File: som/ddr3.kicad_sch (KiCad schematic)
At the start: 10 parts, among them U2 AS4C256M16D3, U3 AS4C256M16D3

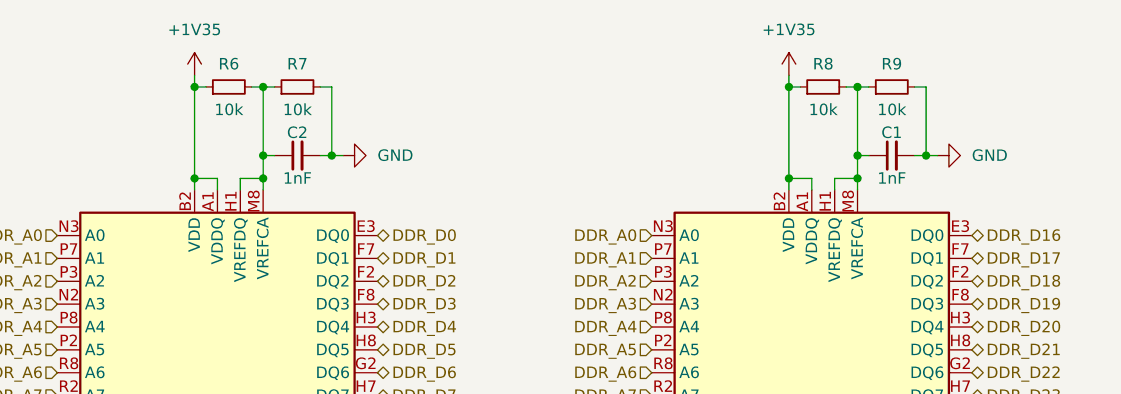
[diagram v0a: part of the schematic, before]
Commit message: DDR3 (again)
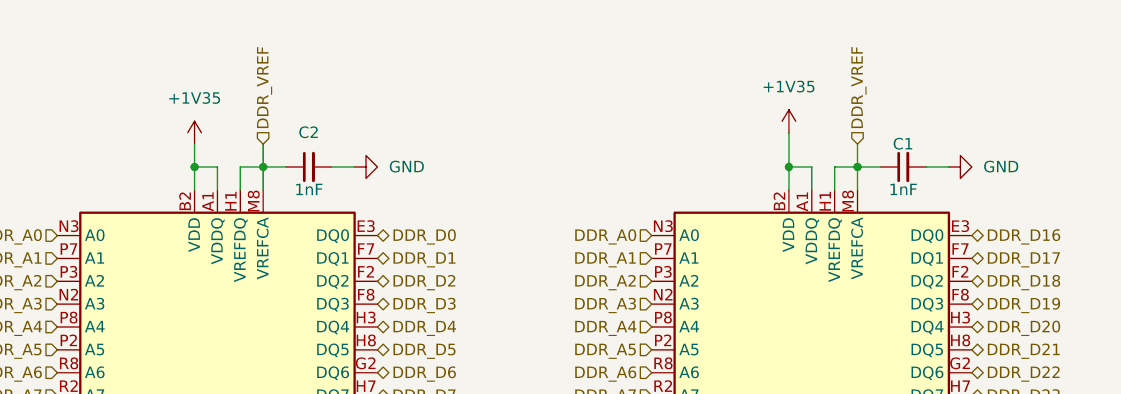
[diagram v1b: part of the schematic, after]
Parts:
- removed R6, R7, R8, R9: 10k, Resistor_SMD:R_0402_1005Metric_Pad0.72x0.64mm_HandSolder, symbol Device:R_Small
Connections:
- net DDR_VREF: now reaches C2.1, U2.H1 (VREFDQ), U2.M8 (VREFCA)
- net DDR_VREF: now also C1.1, U3.H1 (VREFDQ), U3.M8 (VREFCA)
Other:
- moved on the sheet: C1, C2
